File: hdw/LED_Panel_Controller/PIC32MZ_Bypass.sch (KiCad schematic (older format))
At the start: 23 parts

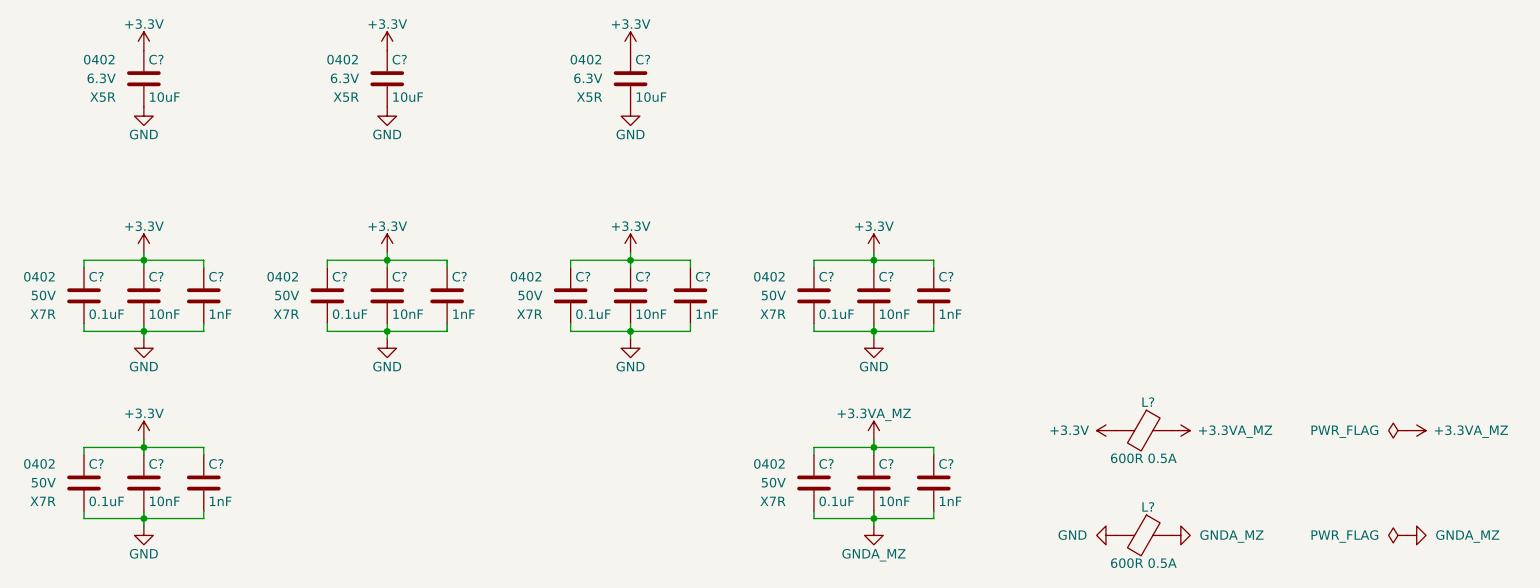
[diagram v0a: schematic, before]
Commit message: Many sch updates
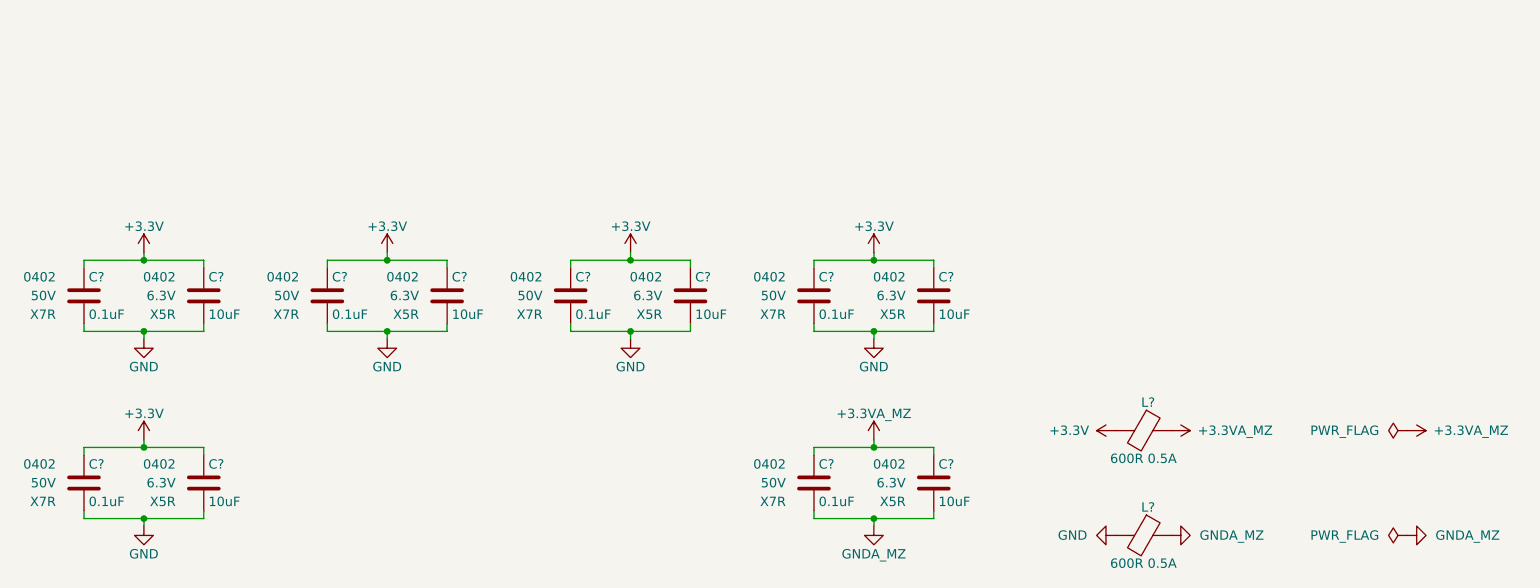
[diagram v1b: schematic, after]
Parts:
- removed C? (x6): 1nF, Capacitors_SMD:C_0402, symbol Custom_Library:C_Custom
- removed C? (x6): 10nF, Capacitors_SMD:C_0402, symbol Custom_Library:C_Custom
- added C? (x3): 10uF, Capacitors_SMD:C_0402, symbol Custom_Library:C_Custom
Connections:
- net +3.3VA_MZ: now also C?.1
- net +3V3: now also C?.1, C?.1
- net GND: now also C?.2, C?.2
- net GNDA_MZ: now also C?.2
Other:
- moved on the sheet: C?
